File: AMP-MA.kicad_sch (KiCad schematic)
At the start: 58 parts, among them J8 Socket_01x05, J9 Socket_01x03, Q1 2N5484, Q2 2N5484, Q3 2N5484, Q4 2N5484, U2 LM1875, U3 TL072

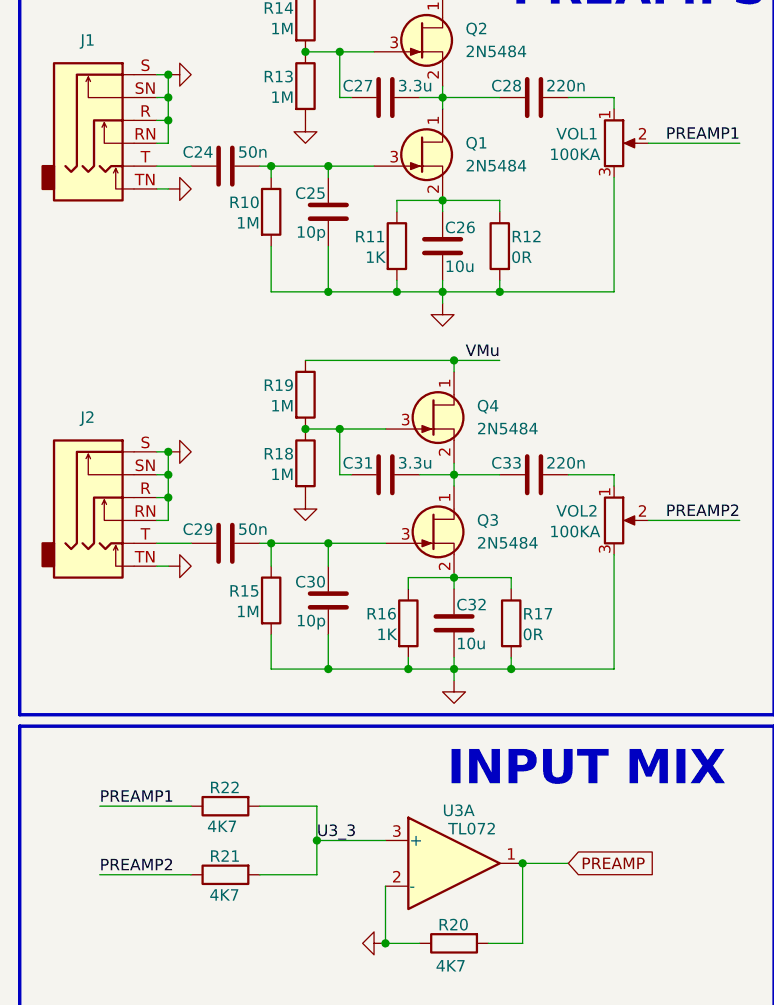
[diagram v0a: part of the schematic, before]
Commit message: Revert "Beta 0.0.1"
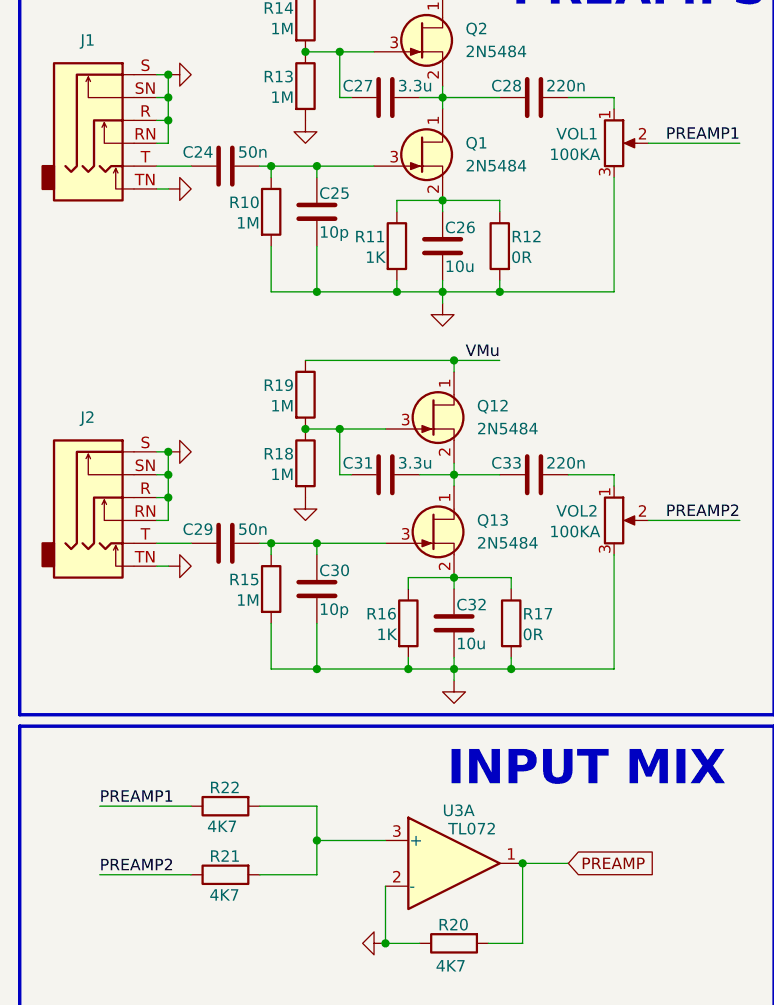
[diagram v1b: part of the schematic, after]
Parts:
- renumbered Q4 to Q12, Q3 to Q13
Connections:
- net U3_3: no longer names the net of R21.2, R22.2, U3.3 (+)
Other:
- moved on the sheet: C25, C30, R15
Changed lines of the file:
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@@
 	)
 	(junction
-		(at 46.99 36.83)
+		(at 45.72 36.83)
 		(diameter 0)
 		(color 0 0 0 0)
@@
 	)
 	(junction
-		(at 46.99 78.74)
+		(at 45.72 78.74)
 		(diameter 0)
 		(color 0 0 0 0)
@@
 	)
 	(junction
-		(at 46.99 50.8)
+		(at 45.72 50.8)
 		(diameter 0)
 		(color 0 0 0 0)
@@
 	)
 	(junction
-		(at 46.99 92.71)
+		(at 45.72 92.71)
 		(diameter 0)
 		(color 0 0 0 0)
@@
 	(wire
 		(pts
+			(xy 45.72 78.74) (xy 53.34 78.74)
+		)
+		(stroke
+			(width 0)
+			(type default)
+		)
+	)
+	(wire
+		(pts
 			(xy 158.75 67.31) (xy 158.75 73.66)
 		)
@@
 	(wire
 		(pts
+			(xy 54.61 50.8) (xy 45.72 50.8)
+		)
+		(stroke
+			(width 0)
+			(type default)
+		)
+	)
+	(wire
+		(pts
 			(xy 59.69 16.51) (xy 59.69 17.78)
 		)
@@
 	(wire
 		(pts
+			(xy 45.72 36.83) (xy 52.07 36.83)
+		)
+		(stroke
+			(width 0)
+			(type default)
+		)
+	)
+	(wire
+		(pts
 			(xy 29.21 71.12) (xy 29.21 73.66)
 		)
@@
 	(wire
 		(pts
-			(xy 40.64 88.9) (xy 40.64 92.71)
+			(xy 40.64 87.63) (xy 40.64 92.71)
 		)
 		(stroke
@@
 	(wire
 		(pts
-			(xy 46.99 38.1) (xy 46.99 36.83)
+			(xy 45.72 38.1) (xy 45.72 36.83)
 		)
 		(stroke
@@
 	(wire
 		(pts
+			(xy 45.72 92.71) (xy 55.88 92.71)
+		)
+		(stroke
+			(width 0)
+			(type default)
+		)
+	)
+	(wire
+		(pts
 			(xy 118.11 95.25) (xy 120.65 95.25)
 		)
@@
 	(wire
 		(pts
-			(xy 40.64 92.71) (xy 55.88 92.71)
+			(xy 40.64 92.71) (xy 45.72 92.71)
 		)
 		(stroke
@@
 	(wire
 		(pts
-			(xy 46.99 81.28) (xy 46.99 78.74)
+			(xy 45.72 80.01) (xy 45.72 78.74)
 		)
 		(stroke
@@
 	(wire
 		(pts
-			(xy 40.64 78.74) (xy 40.64 81.28)
+			(xy 40.64 78.74) (xy 40.64 80.01)
 		)
 		(stroke
@@
 	(wire
 		(pts
-			(xy 46.99 88.9) (xy 46.99 92.71)
+			(xy 45.72 87.63) (xy 45.72 92.71)
 		)
 		(stroke
@@
 	(wire
 		(pts
-			(xy 46.99 45.72) (xy 46.99 50.8)
+			(xy 45.72 45.72) (xy 45.72 50.8)
 		)
 		(stroke
@@
 	(wire
 		(pts
-			(xy 40.64 78.74) (xy 53.34 78.74)
+			(xy 40.64 78.74) (xy 45.72 78.74)
 		)
 		(stroke
@@
 	(wire
 		(pts
-			(xy 40.64 50.8) (xy 54.61 50.8)
+			(xy 40.64 50.8) (xy 45.72 50.8)
 		)
 		(stroke
@@
 	(wire
 		(pts
-			(xy 40.64 36.83) (xy 52.07 36.83)
+			(xy 40.64 36.83) (xy 45.72 36.83)
 		)
 		(stroke
@@
 		)
 	)
-	(label "U3_3"
-		(at 45.72 111.76 0)
-		(effects
-			(font
-				(size 1.27 1.27)
-			)
-			(justify left bottom)
-		)
-	)
 	(label "LM_IN+"
 		(at 121.92 71.12 0)
@@
 	(symbol
 		(lib_id "Device:C")
-		(at 46.99 85.09 0)
-		(mirror x)
+		(at 45.72 83.82 180)
 		(unit 1)
 		(body_style 1)
@@
 		(dnp no)
 		(property "Reference" "C30"
-			(at 46.736 83.058 0)
+			(at 45.974 81.788 0)
 			(show_name no)
 			(do_not_autoplace no)
@@
 		)
 		(property "Value" "10p"
-			(at 46.736 87.376 0)
+			(at 45.974 86.106 0)
 			(show_name no)
 			(do_not_autoplace no)
@@
 		)
 		(property "Footprint" "PrLib:C_disc_D7_W2.5_P5"
-			(at 47.9552 81.28 0)
+			(at 44.7548 80.01 0)
 			(hide yes)
 			(show_name no)
@@
 		)
 		(property "Datasheet" ""
-			(at 46.99 85.09 0)
+			(at 45.72 83.82 0)
 			(hide yes)
 			(show_name no)
@@
 		)
 		(property "Description" "Unpolarized capacitor"
-			(at 46.99 85.09 0)
+			(at 45.72 83.82 0)
 			(hide yes)
 			(show_name no)
@@
 		(dnp no)
 		(fields_autoplaced yes)
-		(property "Reference" "Q3"
+		(property "Reference" "Q13"
 			(at 63.5 76.1999 0)
 			(show_name no)
@@
 			(project "AMP-MA"
 				(path "/4094031b-a9da-4ac5-aaa1-42b342c92a3e"
-					(reference "Q3")
+					(reference "Q13")
 					(unit 1)
 				)
@@
 	(symbol
 		(lib_id "Device:C")
-		(at 46.99 41.91 0)
-		(mirror x)
+		(at 45.72 41.91 180)
 		(unit 1)
 		(body_style 1)
@@
 		(dnp no)
 		(property "Reference" "C25"
-			(at 46.736 39.878 0)
+			(at 45.974 39.878 0)
 			(show_name no)
 			(do_not_autoplace no)
@@
 		)
 		(property "Value" "10p"
-			(at 46.736 44.196 0)
+			(at 45.974 44.196 0)
 			(show_name no)
 			(do_not_autoplace no)
@@
 		)
 		(property "Footprint" "PrLib:C_disc_D7_W2.5_P5"
-			(at 47.9552 38.1 0)
+			(at 44.7548 38.1 0)
 			(hide yes)
 			(show_name no)
@@
 		)
 		(property "Datasheet" ""
-			(at 46.99 41.91 0)
+			(at 45.72 41.91 0)
 			(hide yes)
 			(show_name no)
@@
 		)
 		(property "Description" "Unpolarized capacitor"
-			(at 46.99 41.91 0)
+			(at 45.72 41.91 0)
 			(hide yes)
 			(show_name no)
@@
 	(symbol
 		(lib_id "Device:R")
-		(at 40.64 85.09 0)
+		(at 40.64 83.82 0)
 		(unit 1)
 		(body_style 1)
@@
 		(dnp no)
 		(property "Reference" "R15"
-			(at 39.37 84.074 0)
+			(at 39.37 82.804 0)
 			(show_name no)
 			(do_not_autoplace no)
@@
 		)
 		(property "Value" "1M"
-			(at 39.37 86.36 0)
+			(at 39.37 85.09 0)
 			(show_name no)
 			(do_not_autoplace no)
@@
 		)
 		(property "Footprint" "Resistor_THT:R_Axial_DIN0207_L6.3mm_D2.5mm_P10.16mm_Horizontal"
-			(at 38.862 85.09 90)
+			(at 38.862 83.82 90)
 			(hide yes)
 			(show_name no)
@@
 		)
 		(property "Datasheet" ""
-			(at 40.64 85.09 0)
+			(at 40.64 83.82 0)
 			(hide yes)
 			(show_name no)
@@
 		)
 		(property "Description" "Resistor"
-			(at 40.64 85.09 0)
+			(at 40.64 83.82 0)
 			(hide yes)
 			(show_name no)
@@
 		(dnp no)
 		(fields_autoplaced yes)
-		(property "Reference" "Q4"
+		(property "Reference" "Q12"
 			(at 63.5 63.4999 0)
 			(show_name no)
@@
 			(project "AMP-MA"
 				(path "/4094031b-a9da-4ac5-aaa1-42b342c92a3e"
-					(reference "Q4")
+					(reference "Q12")
 					(unit 1)
 				)
